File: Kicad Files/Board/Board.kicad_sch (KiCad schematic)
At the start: 28 parts, among them SW1 Boot, U1 RP2040, U2 W25Q128JVS, U3 SRV05-4, U4 XC6206PxxxMR, U5 X322512MSB4SI

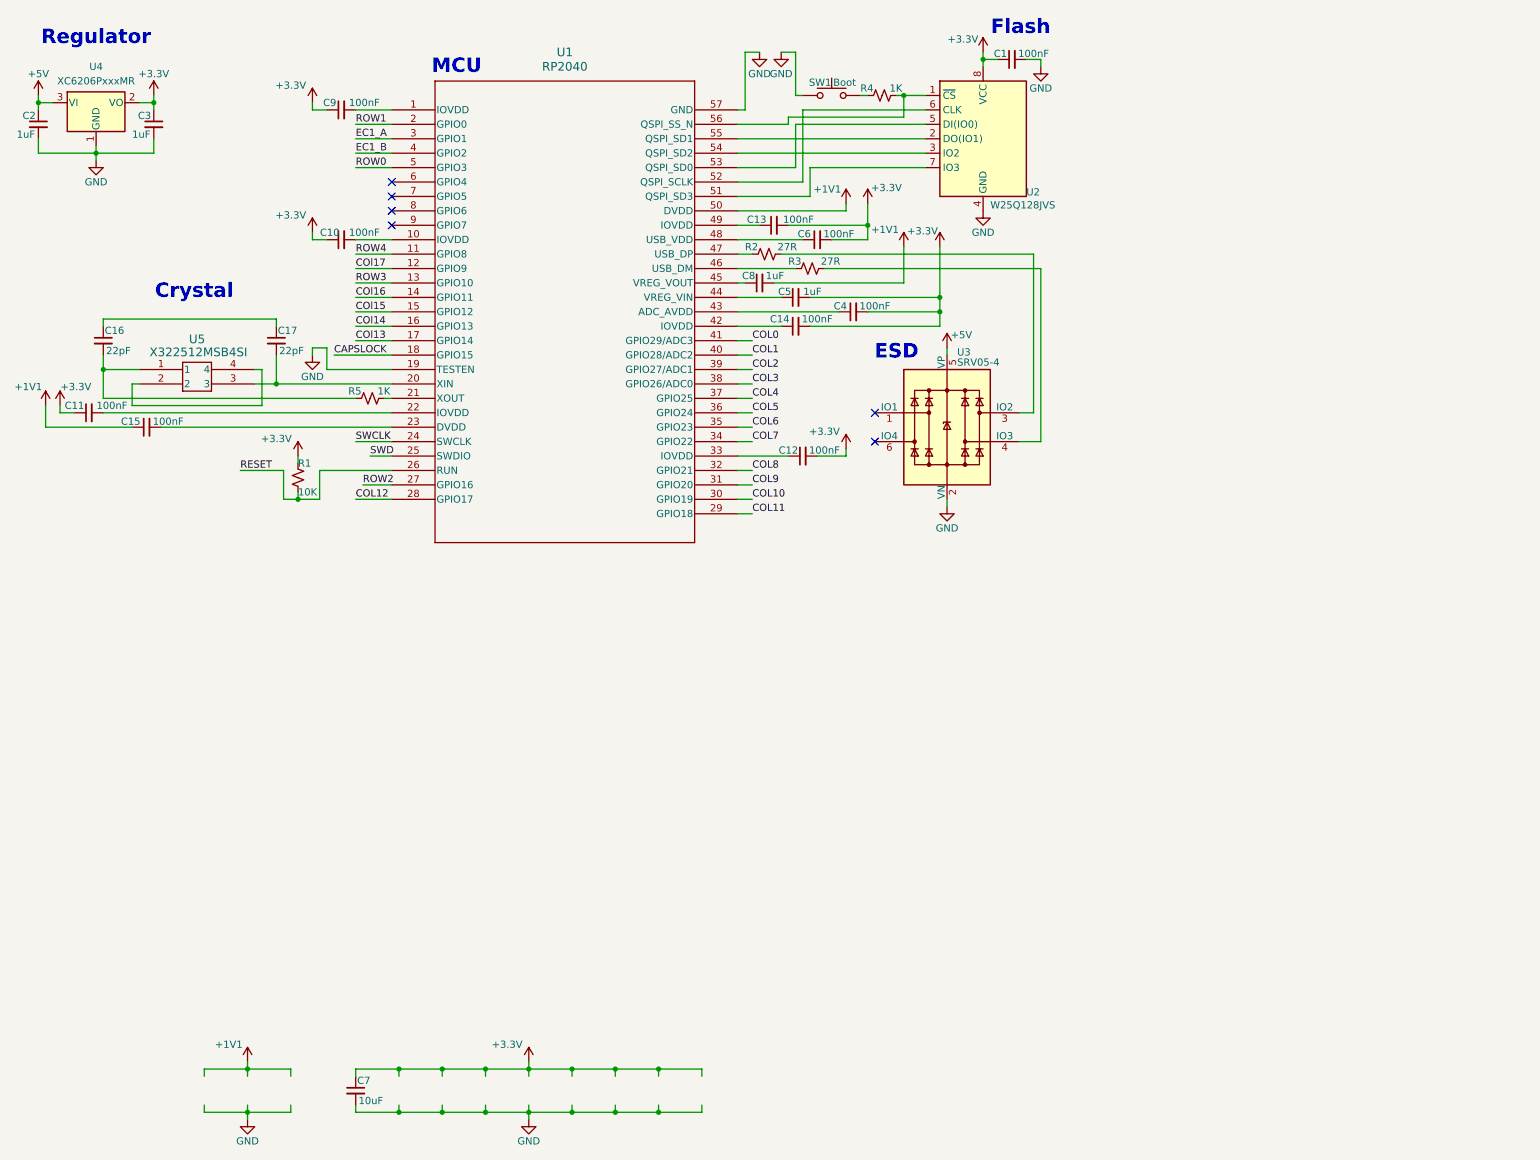
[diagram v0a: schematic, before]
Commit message: Modified Schematic
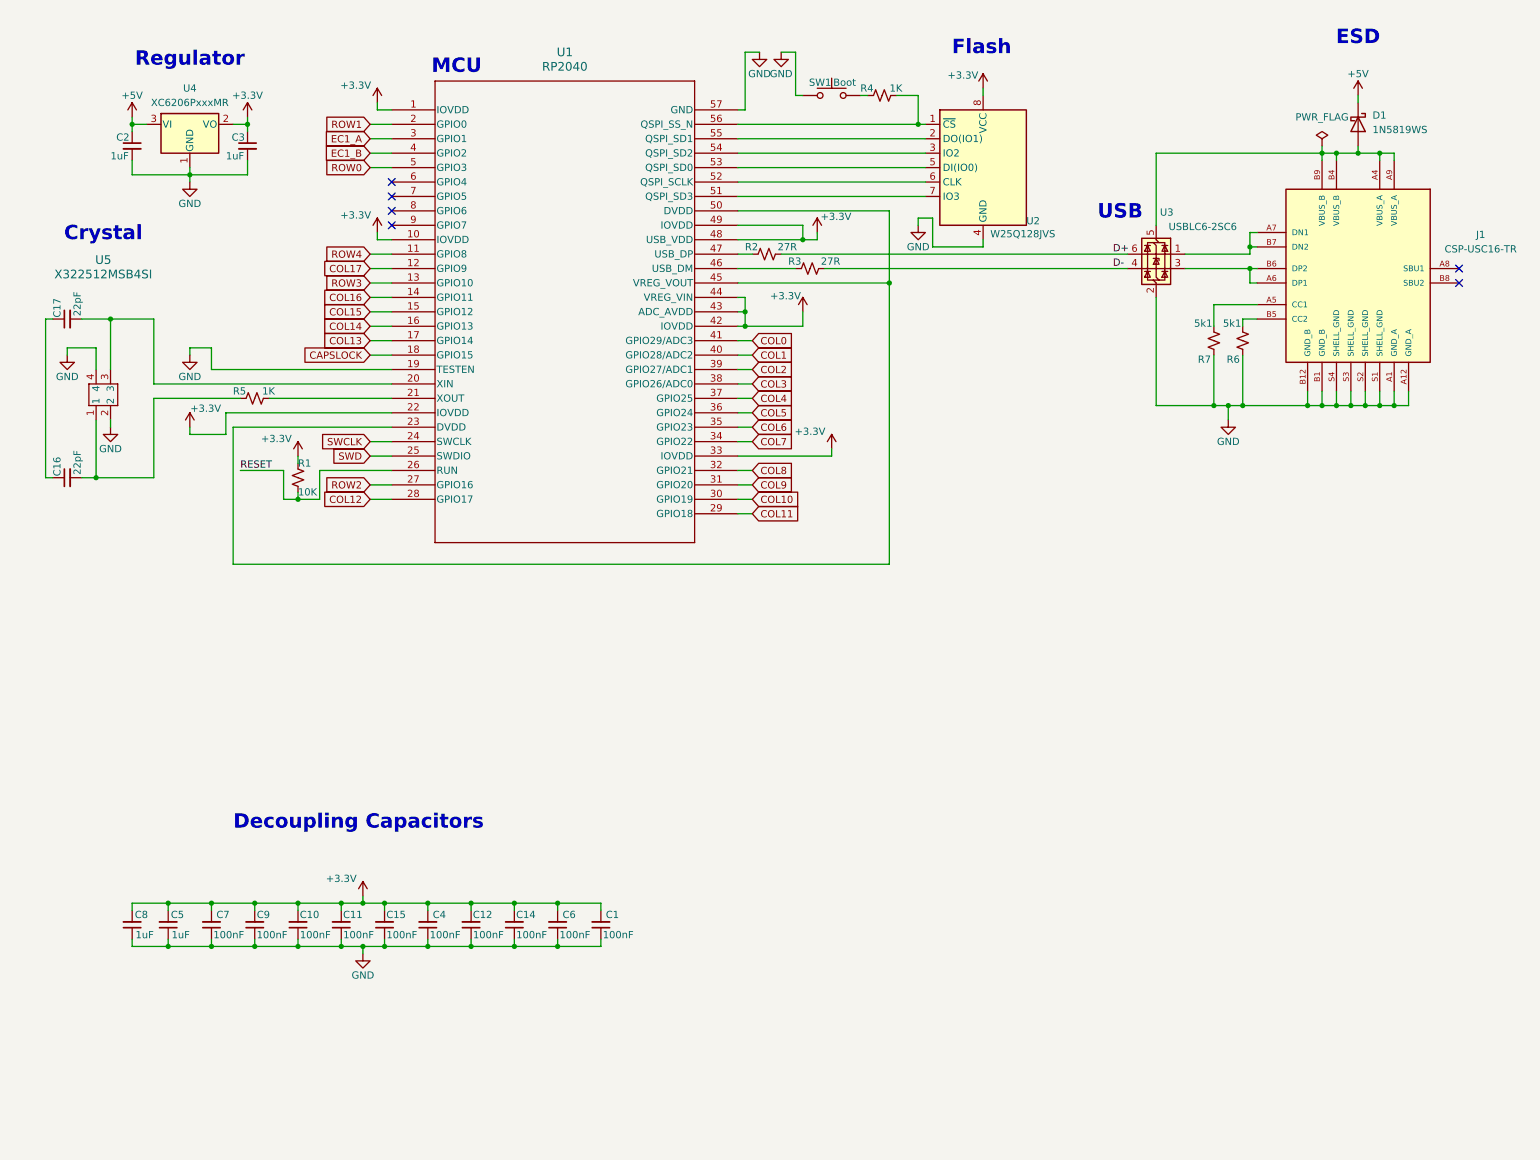
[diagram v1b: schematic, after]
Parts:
- removed C13: 100nF, mechanical_keyboard:C_0402_1005Metric, symbol mechanical_keyboard:C_Small
- removed U3: SRV05-4, mechanical_keyboard:SOT-23-6, symbol mechanical_keyboard:SRV05-4
- added D1: 1N5819WS, mechanical_keyboard:D_SOD-323, symbol mechanical_keyboard:1N5819WS
- added J1: CSP-USC16-TR, mechanical_keyboard:USB_C_Receptacle_HRO_TYPE-C-31-M-12, symbol mechanical_keyboard:CSP-USC16-TR
- added R6, R7: 5k1, mechanical_keyboard:R_0402_1005Metric, symbol Device:R_Small_US
- added U3: USBLC6-2SC6, mechanical_keyboard:SOT-23-6, symbol mechanical_keyboard:USBLC6-2SC6
- C7: value 10uF -> 100nF; LCSC Part # C15525 -> C1525
- U2: footprint mechanical_keyboard:SOIC-8_5.23x5.23mm_P1.27mm -> Package_SO:SOIC-8_5.23x5.23mm_P1.27mm
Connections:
- net +3.3V: now also C1.2, C10.2, C11.2, C15.2, C7.2, C8.2, C9.2, U1.1 (IOVDD), U1.10 (IOVDD), U1.22 (IOVDD), U1.33 (IOVDD), U1.42 (IOVDD), U1.43 (ADC_AVDD), U1.44 (VREG_VIN), U1.48 (USB_VDD), U1.49 (IOVDD); no longer C1.1, C10.1, C11.1, C7.1, C9.1
- net +5V: now also D1.1 (K)
- net GND: now also C1.1, C10.1, C11.1, C12.1, C14.1, C15.1, C4.1, C5.1, C6.1, C7.1, C8.1, C9.1, U5.2, U5.4, J1.A1 (GND_A), J1.A12 (GND_A), J1.B1 (GND_B), J1.B12 (GND_B), J1.S1 (SHELL_GND), J1.S2 (SHELL_GND), J1.S3 (SHELL_GND), J1.S4 (SHELL_GND), R6.1, R7.1, U3.2 (GND); no longer C1.2, C7.2
- net at U1.23 (DVDD): now also U1.45 (VREG_VOUT), U1.50 (DVDD); no longer C15.2
- net D+: now reaches R2.2
- net D+: now also U3.6 (I/O1)
- net D-: now reaches R3.2
- net D-: now also U3.4 (I/O2)
- removed net +1V1: C15.1, C8.2, U1.50 (DVDD)
- net COl13 renamed COL13
- net COl14 renamed COL14
- net COl15 renamed COL15
- net COl16 renamed COL16
- net COl17 renamed COL17
- new net: J1.A5 (CC1), R7.2
- new net: J1.A7 (DN1), J1.B7 (DN2), U3.1 (I/O1)
- new net: J1.A6 (DP1), J1.B6 (DP2), U3.3 (I/O2)
- new net: D1.2 (A), J1.A4 (VBUS_A), J1.A9 (VBUS_A), J1.B4 (VBUS_B), J1.B9 (VBUS_B), U3.5 (VBUS)
- new net: J1.B5 (CC2), R6.2
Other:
- note added: "Decoupling Capacitors"
- note added: "USB"
- moved on the sheet: C16, C17, C2, C3, R5, U2, U4, U5
